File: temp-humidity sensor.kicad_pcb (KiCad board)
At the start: 2 copper layers, 75 x 31.5 mm, 45 parts, among them J1 Conn_01x02, J2 USB_C_Receptacle_USB2.0_16P, SW1 SW_Push, SW2 SW_Push, U1 SHT4x, U2 ESP32-C6-WROOM-1, U3 BQ24074RGT, U4 USBLC6-2SC6, U5 TPS63031DSK, U6 SS12D10G5

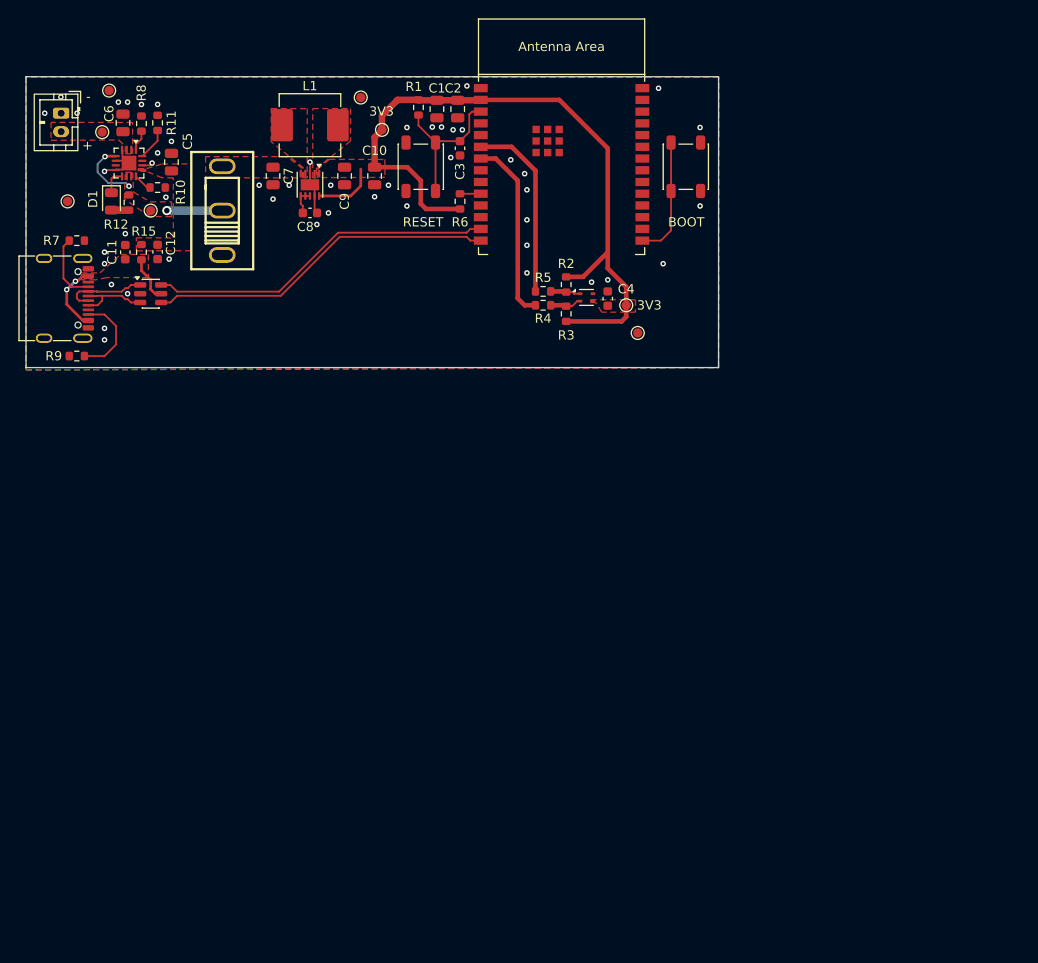
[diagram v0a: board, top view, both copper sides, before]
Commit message: Improved design
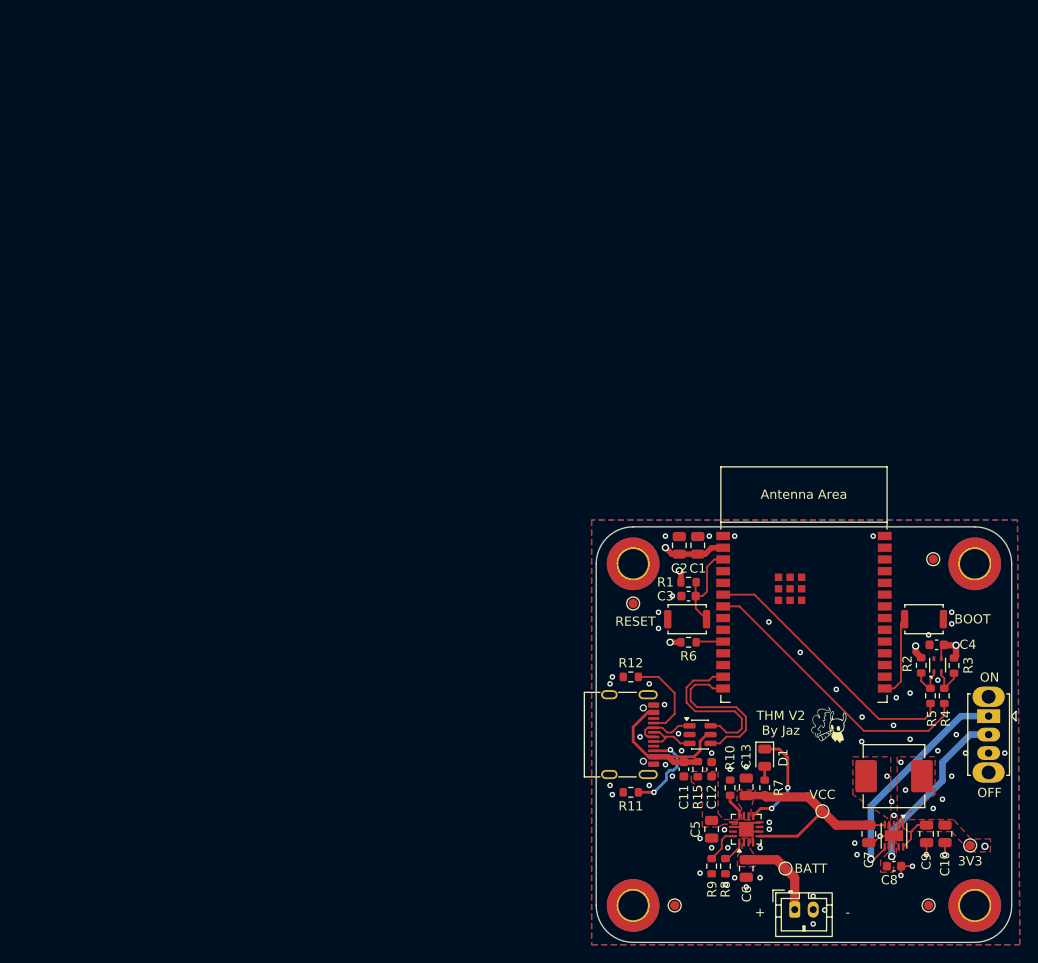
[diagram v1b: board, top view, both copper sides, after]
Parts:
- removed TP4: TestPoint, TestPoint:TestPoint_Pad_D1.0mm
- removed U6: SS12D10G5, easyeda2kicad:SW-TH_SHOU-HAN_SS12D10G4
- added C13: 4.7u, Capacitor_SMD:C_0805_2012Metric, F.Cu at (143.2, 113.7)
- added G***: LOGO, LOGO, F.Cu at (152.2, 107.0)
- added G***: LOGO, LOGO, B.Cu at (149.0, 95.0)
- added H1: MountingHole, MountingHole:MountingHole_3.2mm_M3_ISO7380_Pad_TopBottom, F.Cu at (131.0, 89.5)
- added H2: MountingHole, MountingHole:MountingHole_3.2mm_M3_ISO7380_Pad_TopBottom, F.Cu at (131.0, 126.5)
- added H3: MountingHole, MountingHole:MountingHole_3.2mm_M3_ISO7380_Pad_TopBottom, F.Cu at (168.0, 126.5)
- added H4: MountingHole, MountingHole:MountingHole_3.2mm_M3_ISO7380_Pad_TopBottom, F.Cu at (168.0, 89.5)
- added SW3: SW_SPDT, Button_Switch_THT:SW_Slide_SPDT_Straight_CK_OS102011MS2Q, F.Cu at (169.5, 106.0)
- SW1, SW2: footprint Button_Switch_SMD:SW_SPST_PTS647_Sx38 -> Button_Switch_SMD:SW_Push_SPST_NO_Alps_SKRK
- moved J1 117.3 mm to (148.5, 127.0), turned to 0 degrees
- moved TP5 108.8 mm to (147.5, 122.5), turned to 0 degrees
- moved TP7 107.0 mm to (163.0, 126.5)
- moved C6 105.2 mm to (143.2, 122.5), turned to -90 degrees
- moved TP6 102.7 mm to (163.5, 89.0), turned to 180 degrees
- moved R8 102.3 mm to (141.0, 122.2), turned to -90 degrees
- moved TP9 100.7 mm to (135.5, 126.5), turned to 180 degrees
- moved R9 100.4 mm to (139.5, 122.2), turned to 90 degrees
- moved U3 98.4 mm to (143.2, 118.2), turned to 90 degrees
- moved TP3 97.6 mm to (151.5, 116.3), turned to 0 degrees
- moved C7 96.1 mm to (156.5, 118.8)
- moved C9 95.1 mm to (162.8, 118.8)
- moved C8 94.9 mm to (159.2, 122.2)
- moved L1 94.7 mm to (159.2, 112.5)
- moved U5 94.7 mm to (159.2, 119.0)
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- renumbered R9 to R11, R7 to R12, R12 to R7, R11 to R9
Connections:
- C7 pad 1: /VIN -> VCC
- C8 pad 1: Net-(U5-EN) -> VINA
- J1 pad 1: Earth -> /BAT+
- J1 pad 2: /BAT+ -> Earth
- U5 pad 5: /VIN -> VCC
- U5 pad 6: Net-(U5-EN) -> PWR_EN
- U5 pad 7: Net-(U5-EN) -> VINA
- U5 pad 8: Net-(U5-EN) -> VINA
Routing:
- net +3V3: track 84.1 -> 19.3 mm, vias 0 -> 6
- net PWR_EN: track 0.00 -> 24.7 mm, vias 0 -> 1
- net USBD+: track 37.7 -> 18.1 mm
- net USBD-: track 37.7 -> 18.1 mm
- net VINA: track 0.00 -> 18.7 mm, vias 0 -> 1
- net SCL: track 20.0 -> 31.5 mm
- net VCC: track 13.2 -> 24.3 mm, vias 3 -> 0
- net /BAT+: track 0.00 -> 9.51 mm
- net SDA: track 20.1 -> 29.3 mm
- net Net-(D1-K): track 2.77 -> 11.4 mm, vias 0 -> 2
- net /VBUS: track 12.6 -> 20.2 mm, vias 2 -> 0
- net CHIP_PU: track 16.5 -> 10.7 mm
- net GPIO9: track 13.1 -> 8.98 mm
- net Net-(U5-EN): track 3.25 -> 0.00 mm
- net /USBCD-: track 9.13 -> 6.96 mm
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- added copper zone on In2.Cu, net +3V3
- added copper zone on In1.Cu, net Earth
- added copper zone on F.Cu, net VINA
- removed copper zone on F.Cu, net /VBUS
- removed copper zone on F.Cu, net /VIN
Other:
- board size 75 x 31.5 mm -> 45 x 45 mm
- copper layers 2 -> 4
- board text added: "BATT"
- board text added: "OFF"
- board text added: "ON"
- board text added: "THM V2 By Jaz"
- board text added: "VCC"
